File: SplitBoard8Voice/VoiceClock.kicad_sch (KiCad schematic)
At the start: 26 parts, among them U1001 4013, U1002 74HC595, U1003 4013, U1004 74LS08, U1005 74HC595

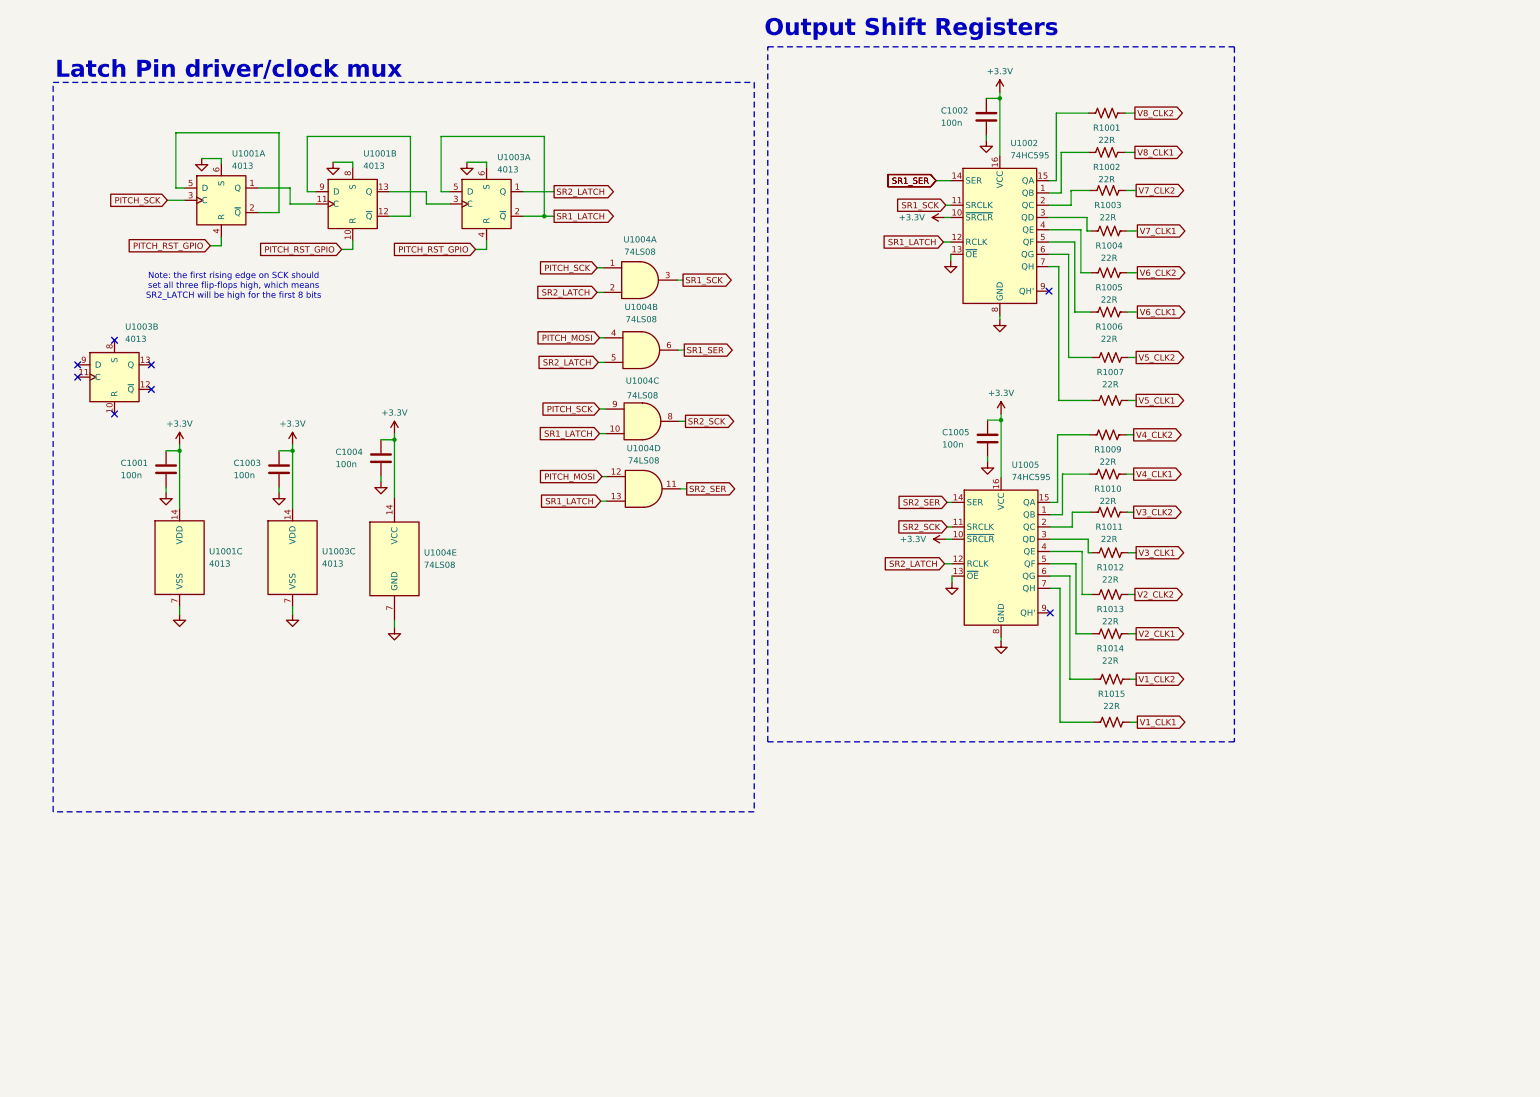
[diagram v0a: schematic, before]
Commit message: galaxy brain clock logic circuit
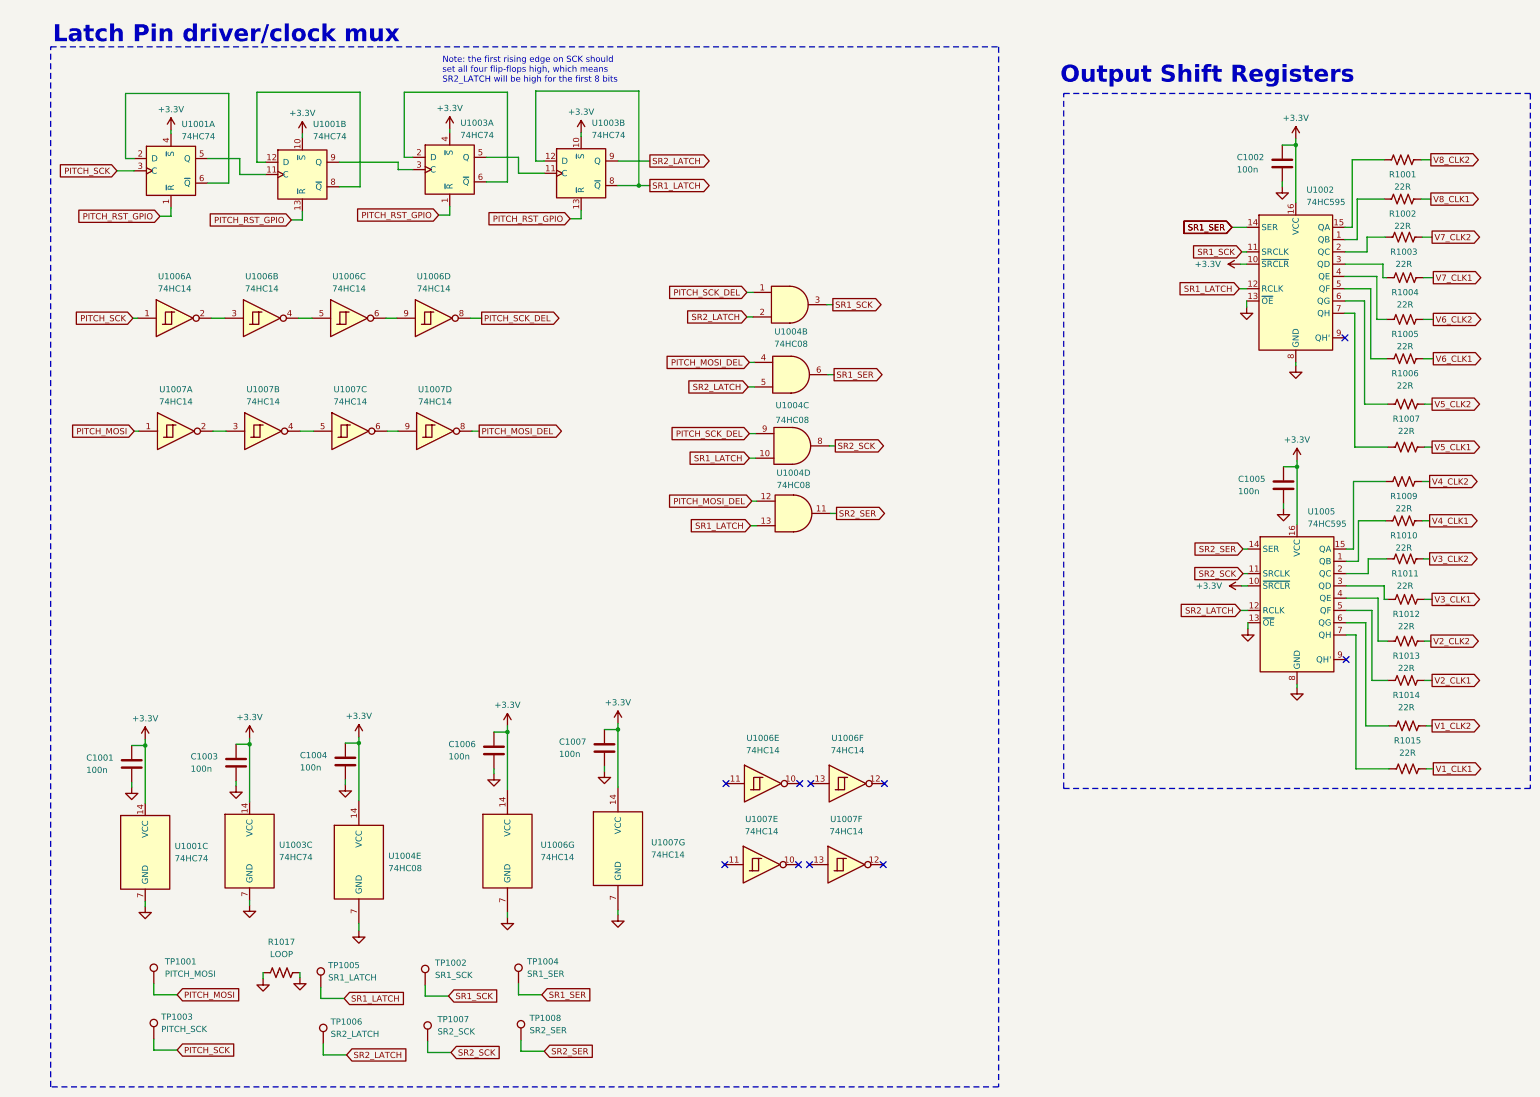
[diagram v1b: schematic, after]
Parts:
- removed U1001, U1003: 4013, symbol 4xxx:4013
- added C1006, C1007: 100n, Capacitor_SMD:C_0805_2012Metric, symbol Device:C
- added R1017: LOOP, Resistor_THT:R_Axial_DIN0204_L3.6mm_D1.6mm_P5.08mm_Horizontal, symbol Device:R_US
- added TP1001: PITCH_MOSI, TestPoint:TestPoint_THTPad_D1.0mm_Drill0.5mm_VAL, symbol Connector:TestPoint
- added TP1002: SR1_SCK, TestPoint:TestPoint_THTPad_D1.0mm_Drill0.5mm_VAL, symbol Connector:TestPoint
- added TP1003: PITCH_SCK, TestPoint:TestPoint_THTPad_D1.0mm_Drill0.5mm_VAL, symbol Connector:TestPoint
- added TP1004: SR1_SER, TestPoint:TestPoint_THTPad_D1.0mm_Drill0.5mm_VAL, symbol Connector:TestPoint
- added TP1005: SR1_LATCH, TestPoint:TestPoint_THTPad_D1.0mm_Drill0.5mm_VAL, symbol Connector:TestPoint
- added TP1006: SR2_LATCH, TestPoint:TestPoint_THTPad_D1.0mm_Drill0.5mm_VAL, symbol Connector:TestPoint
- added TP1007: SR2_SCK, TestPoint:TestPoint_THTPad_D1.0mm_Drill0.5mm_VAL, symbol Connector:TestPoint
- added TP1008: SR2_SER, TestPoint:TestPoint_THTPad_D1.0mm_Drill0.5mm_VAL, symbol Connector:TestPoint
- added U1001, U1003: 74HC74, Package_SO:SOIC-14_3.9x8.7mm_P1.27mm, symbol 74xx:74HC74
- added U1006, U1007: 74HC14, symbol 74xx:74HC14
- U1004: value 74LS08 -> 74HC08; footprint (none) -> Package_SO:SOIC-14_3.9x8.7mm_P1.27mm
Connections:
- net +3.3V: now also C1006.1, C1007.1, U1001.10 (~{S}), U1001.14 (VCC), U1001.4 (~{S}), U1003.10 (~{S}), U1003.14 (VCC), U1003.4 (~{S}), U1006.14 (VCC), U1007.14 (VCC)
- net GND: now also C1006.2, C1007.2, R1017.1, R1017.2, U1001.7 (GND), U1003.7 (GND), U1006.7 (GND), U1007.7 (GND)
- net PITCH_MOSI: now also TP1001.1, U1007.1; no longer U1004.12, U1004.4
- net PITCH_RST_GPIO: now also U1001.1 (~{R}), U1001.13 (~{R}), U1003.1 (~{R}), U1003.13 (~{R})
- net PITCH_SCK: now also TP1003.1, U1001.3 (C), U1006.1; no longer U1004.1, U1004.9
- net SR1_LATCH: now also TP1005.1, U1003.12 (D), U1003.8 (~{Q})
- net SR1_SCK: now also TP1002.1
- net SR1_SER: now also TP1004.1
- net SR2_LATCH: now also TP1006.1, U1003.9 (Q)
- net SR2_SCK: now also TP1007.1
- net SR2_SER: now also TP1008.1
- new net: U1006.2, U1006.3
- new net: U1006.4, U1006.5
- new net: U1003.2 (D), U1003.6 (~{Q})
- new net: U1001.9 (Q), U1003.3 (C)
- new net: U1003.11 (C), U1003.5 (Q)
- new net: U1007.2, U1007.3
- new net: U1007.4, U1007.5
- new net: U1007.6, U1007.9
- new net: U1001.11 (C), U1001.5 (Q)
- new net: U1001.12 (D), U1001.8 (~{Q})
- new net: U1001.2 (D), U1001.6 (~{Q})
- new net: U1006.6, U1006.9
- new net PITCH_MOSI_DEL: U1004.12, U1004.4, U1007.8
- new net PITCH_SCK_DEL: U1004.1, U1004.9, U1006.8
- no-connect marks 8 -> 10
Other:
- note added: "Note: the first rising edge on SCK should set all four flip-flops high, which means SR2_LATCH will be high for the first 8 bits"
- note removed: "Note: the first rising edge on SCK should set all three flip-flops high, which means SR2_LATCH will be high for the first 8 bits"
- moved on the sheet: C1002, C1004, C1005, R1001, R1002, R1003, R1004, R1005, R1006, R1007, R1009, R1010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
